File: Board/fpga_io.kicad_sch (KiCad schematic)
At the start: 2 parts, among them IC1 74LVC125, U4 XC6SLX25-CSG324

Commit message: more layout work
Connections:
- net RAMA9: now also U4.T9 (IO_L32P_GCLK29_2); no longer U4.V6 (IO_L45N_2)
- net HPD_SRC: now reaches U4.K3 (IO_L42N_GCLK24_M3LDM_3)
- net I2C_SCL: now reaches U4.L3 (IO_L39N_M3LDQSN_3)
- net I2C_SDA: now reaches U4.N4 (IO_L1P_3)
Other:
- note added: "(C) A. Fachat"
- note added: "CSA-ULTRACPU-V2.0A-20260906"
- note added: "CSA-ULTRACPU-V3.0A"
- moved on the sheet: IC1A, IC1B, U4A, U4B

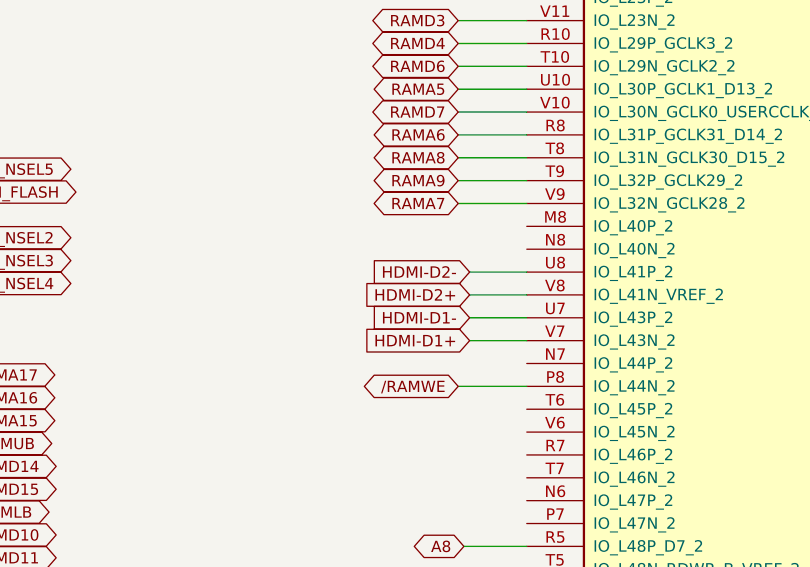
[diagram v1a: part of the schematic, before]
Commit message: more layout work, first candidate
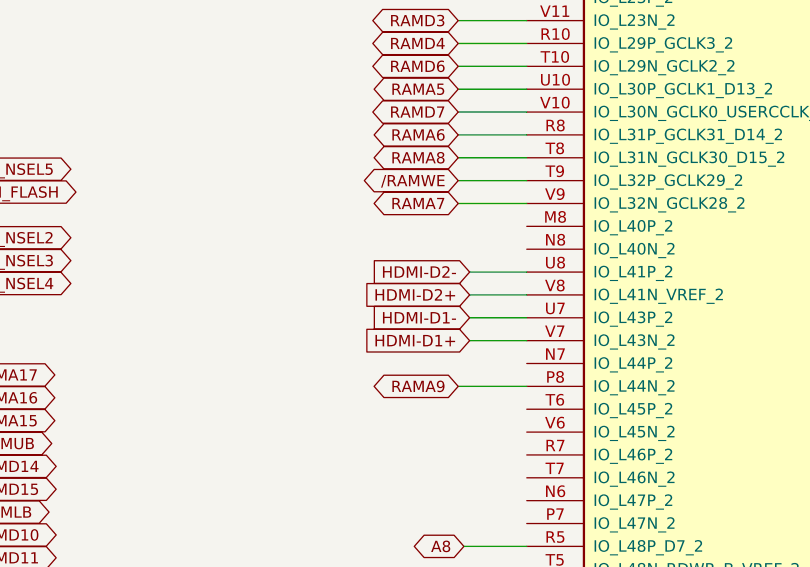
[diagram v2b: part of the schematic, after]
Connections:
- net /RAMWE: now also U4.T9 (IO_L32P_GCLK29_2); no longer U4.P8 (IO_L44N_2)
- net RAMA9: now also U4.P8 (IO_L44N_2); no longer U4.T9 (IO_L32P_GCLK29_2)
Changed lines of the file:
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@@
 	(wire
 		(pts
-			(xy 236.855 190.5) (xy 244.475 190.5)
-		)
-		(stroke
-			(width 0)
-			(type default)
-		)
-	)
-	(wire
-		(pts
 			(xy 172.72 201.93) (xy 181.61 201.93)
 		)
@@
 	(wire
 		(pts
+			(xy 236.855 190.5) (xy 244.475 190.5)
+		)
+		(stroke
+			(width 0)
+			(type default)
+		)
+	)
+	(wire
+		(pts
 			(xy 236.855 162.56) (xy 244.475 162.56)
 		)
@@
 	(wire
 		(pts
-			(xy 236.855 167.64) (xy 244.475 167.64)
-		)
-		(stroke
-			(width 0)
-			(type default)
-		)
-	)
-	(wire
-		(pts
 			(xy 236.855 119.38) (xy 244.475 119.38)
 		)
@@
 	(wire
 		(pts
+			(xy 236.855 167.64) (xy 244.475 167.64)
+		)
+		(stroke
+			(width 0)
+			(type default)
+		)
+	)
+	(wire
+		(pts
 			(xy 236.855 93.98) (xy 244.475 93.98)
 		)
@@
 	(global_label "/RAMWE"
 		(shape bidirectional)
-		(at 236.855 190.5 180)
+		(at 236.855 167.64 180)
 		(fields_autoplaced yes)
 		(effects
@@
 		)
 		(property "Intersheetrefs" "${INTERSHEET_REFS}"
-			(at 225.2546 190.5 0)
+			(at 225.2546 167.64 0)
 			(hide yes)
 			(show_name no)
@@
 	(global_label "RAMA9"
 		(shape bidirectional)
-		(at 236.855 167.64 180)
+		(at 236.855 190.5 180)
 		(fields_autoplaced yes)
 		(effects
@@
 		)
 		(property "Intersheetrefs" "${INTERSHEET_REFS}"
-			(at 226.8549 167.64 0)
+			(at 226.8549 190.5 0)
 			(hide yes)
 			(show_name no)
